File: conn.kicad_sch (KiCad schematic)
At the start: 6 parts, among them J2 Conn_01x04_Pin, J8 USB_C_Receptacle_USB2.0_16P, U12 SRV05-4

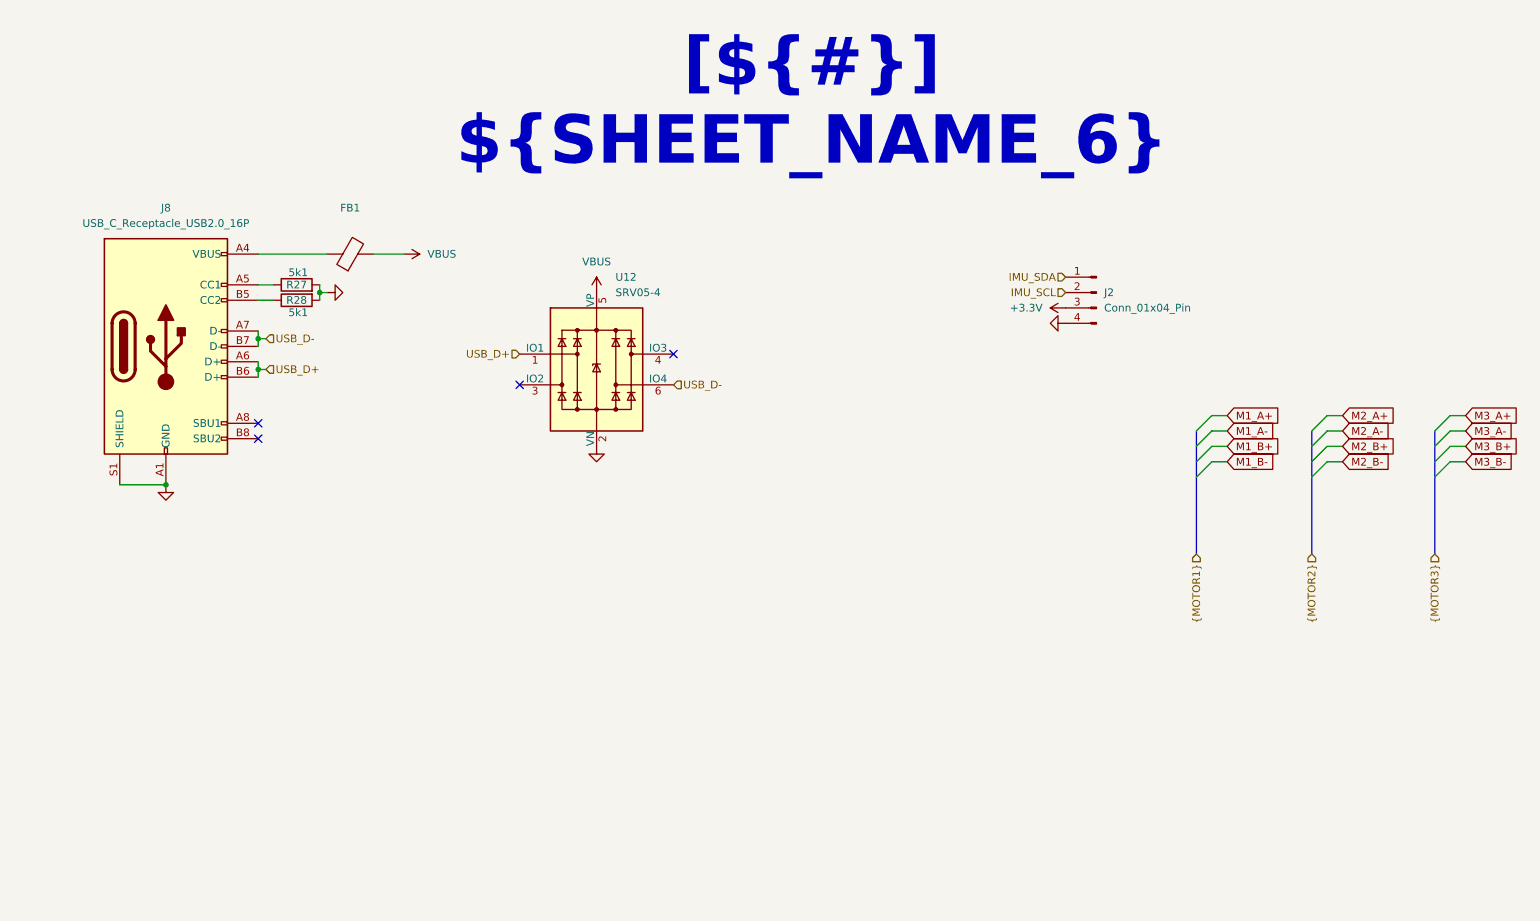
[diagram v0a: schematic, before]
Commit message: Finished design
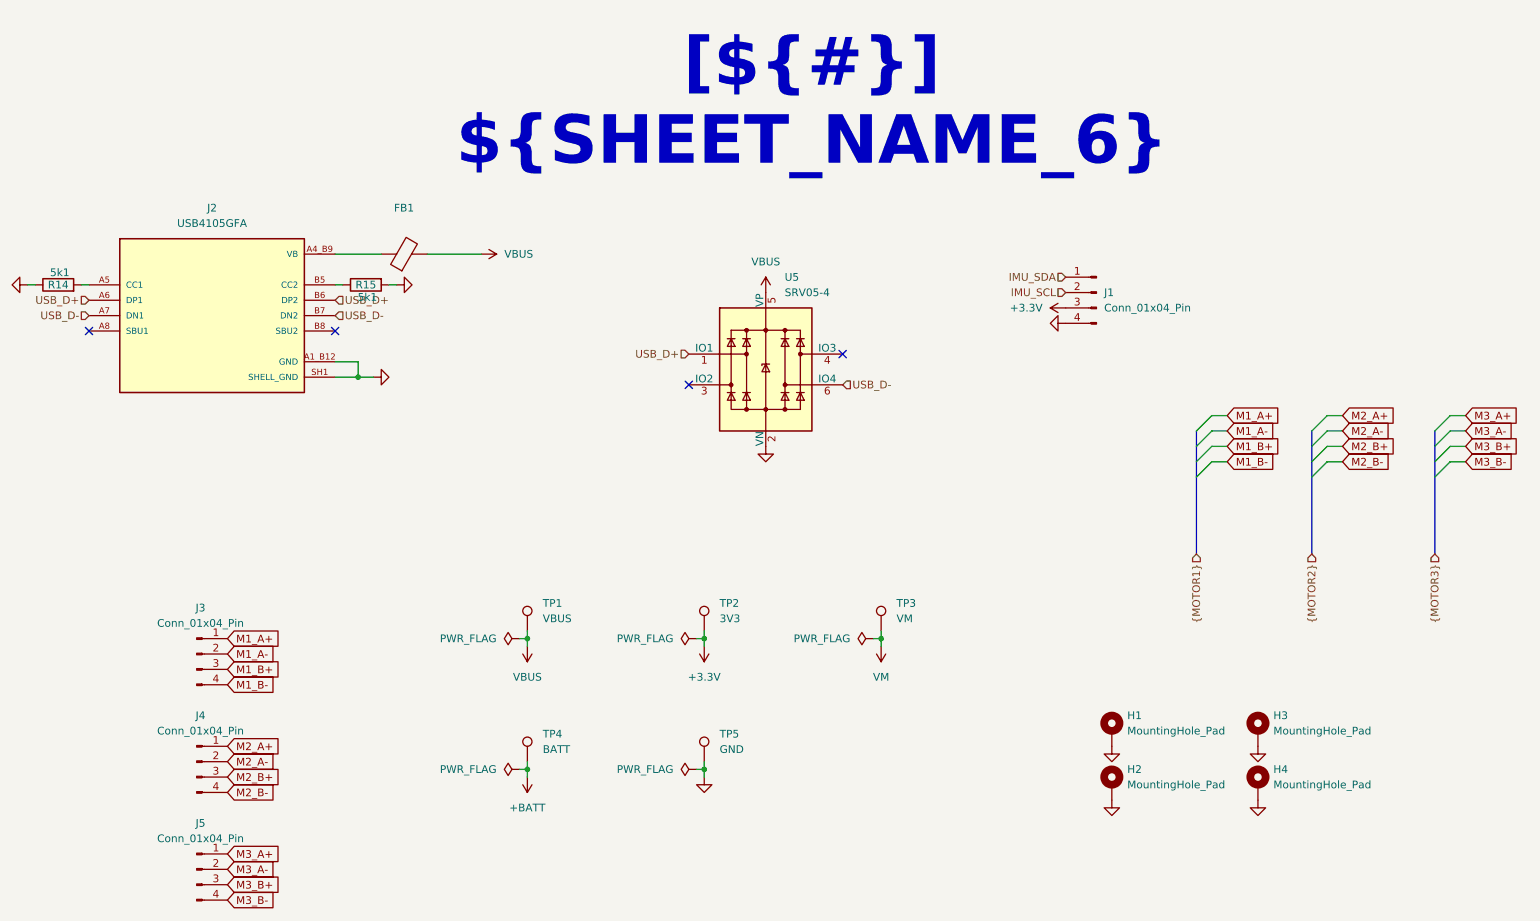
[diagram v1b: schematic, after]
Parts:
- removed J8: USB_C_Receptacle_USB2.0_16P, Connector_USB:USB_C_Receptacle_GCT_USB4105-xx-A_16P_TopMnt_Horizontal, symbol Connector:USB_C_Receptacle_USB2.0_16P
- added H1, H2, H3, H4: MountingHole_Pad, MountingHole:MountingHole_3.2mm_M3_DIN965_Pad, symbol Mechanical:MountingHole_Pad
- added J2: USB4105GFA, Project_Components:GCT_USB4105GFA, symbol Project_Components:USB4105GFA
- added J3, J4, J5: Conn_01x04_Pin, Connector_JST:JST_XH_B4B-XH-A_1x04_P2.50mm_Vertical, symbol Connector:Conn_01x04_Pin
- added TP1: VBUS, TestPoint:TestPoint_Pad_D1.5mm, symbol Connector:TestPoint
- added TP2: 3V3, TestPoint:TestPoint_Pad_D1.5mm, symbol Connector:TestPoint
- added TP3: VM, TestPoint:TestPoint_Pad_D1.5mm, symbol Connector:TestPoint
- added TP4: BATT, TestPoint:TestPoint_Pad_D1.5mm, symbol Connector:TestPoint
- added TP5: GND, TestPoint:TestPoint_Pad_D1.5mm, symbol Connector:TestPoint
- FB1: footprint Inductor_SMD:L_1206_3216Metric_Pad1.22x1.90mm_HandSolder -> Inductor_SMD:L_0603_1608Metric_Pad1.05x0.95mm_HandSolder
- J1: renamed from J2; footprint (none) -> Connector_PinHeader_2.54mm:PinHeader_1x04_P2.54mm_Vertical
- R14: renamed from R27; footprint Resistor_SMD:R_1206_3216Metric_Pad1.30x1.75mm_HandSolder -> Resistor_SMD:R_0603_1608Metric_Pad0.98x0.95mm_HandSolder
- R15: renamed from R28; footprint Resistor_SMD:R_1206_3216Metric_Pad1.30x1.75mm_HandSolder -> Resistor_SMD:R_0603_1608Metric_Pad0.98x0.95mm_HandSolder
- renumbered U12 to U5
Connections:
- net +3.3V: now also TP2.1
- net GND: now also R14.1, H1.1, H2.1, H3.1, H4.1, J2.A1_B12 (GND), J2.B1_A12 (GND), J2.SH1 (SHELL_GND), J2.SH2 (SHELL_GND), J2.SH3 (SHELL_GND), J2.SH4 (SHELL_GND), TP5.1; no longer R14.2
- net M1_A+: now also J3.1 (Pin_1)
- net M1_A-: now also J3.2 (Pin_2)
- net M1_B+: now also J3.3 (Pin_3)
- net M1_B-: now also J3.4 (Pin_4)
- net M2_A+: now also J4.1 (Pin_1)
- net M2_A-: now also J4.2 (Pin_2)
- net M2_B+: now also J4.3 (Pin_3)
- net M2_B-: now also J4.4 (Pin_4)
- net M3_A+: now also J5.1 (Pin_1)
- net M3_A-: now also J5.2 (Pin_2)
- net M3_B+: now also J5.3 (Pin_3)
- net M3_B-: now also J5.4 (Pin_4)
- net USB_D+: now also J2.A6 (DP1), J2.B6 (DP2)
- net USB_D-: now also J2.A7 (DN1), J2.B7 (DN2)
- net VBUS: now also TP1.1
- net VB: now reaches FB1.1
- net VB: now also J2.A4_B9 (VB), J2.B4_A9 (VB)
- net at R15.1: now also J2.B5 (CC2)
- new net: J2.A5 (CC1), R14.2
- new net +BATT: TP4.1
- new net VM: TP3.1
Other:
- moved on the sheet: FB1, R14, R15, U5
